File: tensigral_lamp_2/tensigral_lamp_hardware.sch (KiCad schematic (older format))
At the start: 95 parts, among them J1 USB_B_Micro, J2 JTAG, J3 DEVHDR, J4 WSOUT, J5 VPPS, J6 MICJ, J7 VDDS, J8 WS_SEL, P1 WSIN, P10 AUXTOUCH, P2 WSOUT, P3 VLED, P4 VLED, P5 GND, P6 GND, P9 TOPTOUCH, Q1 3404, Q2 3404, SW1 BOOT0, T1 TOUCH1, T2 TOUCH2, U1 STM32F042F4Px, U2 MT2492, U3 NUP4202, U4 XC6206P360MR, U5 LM321

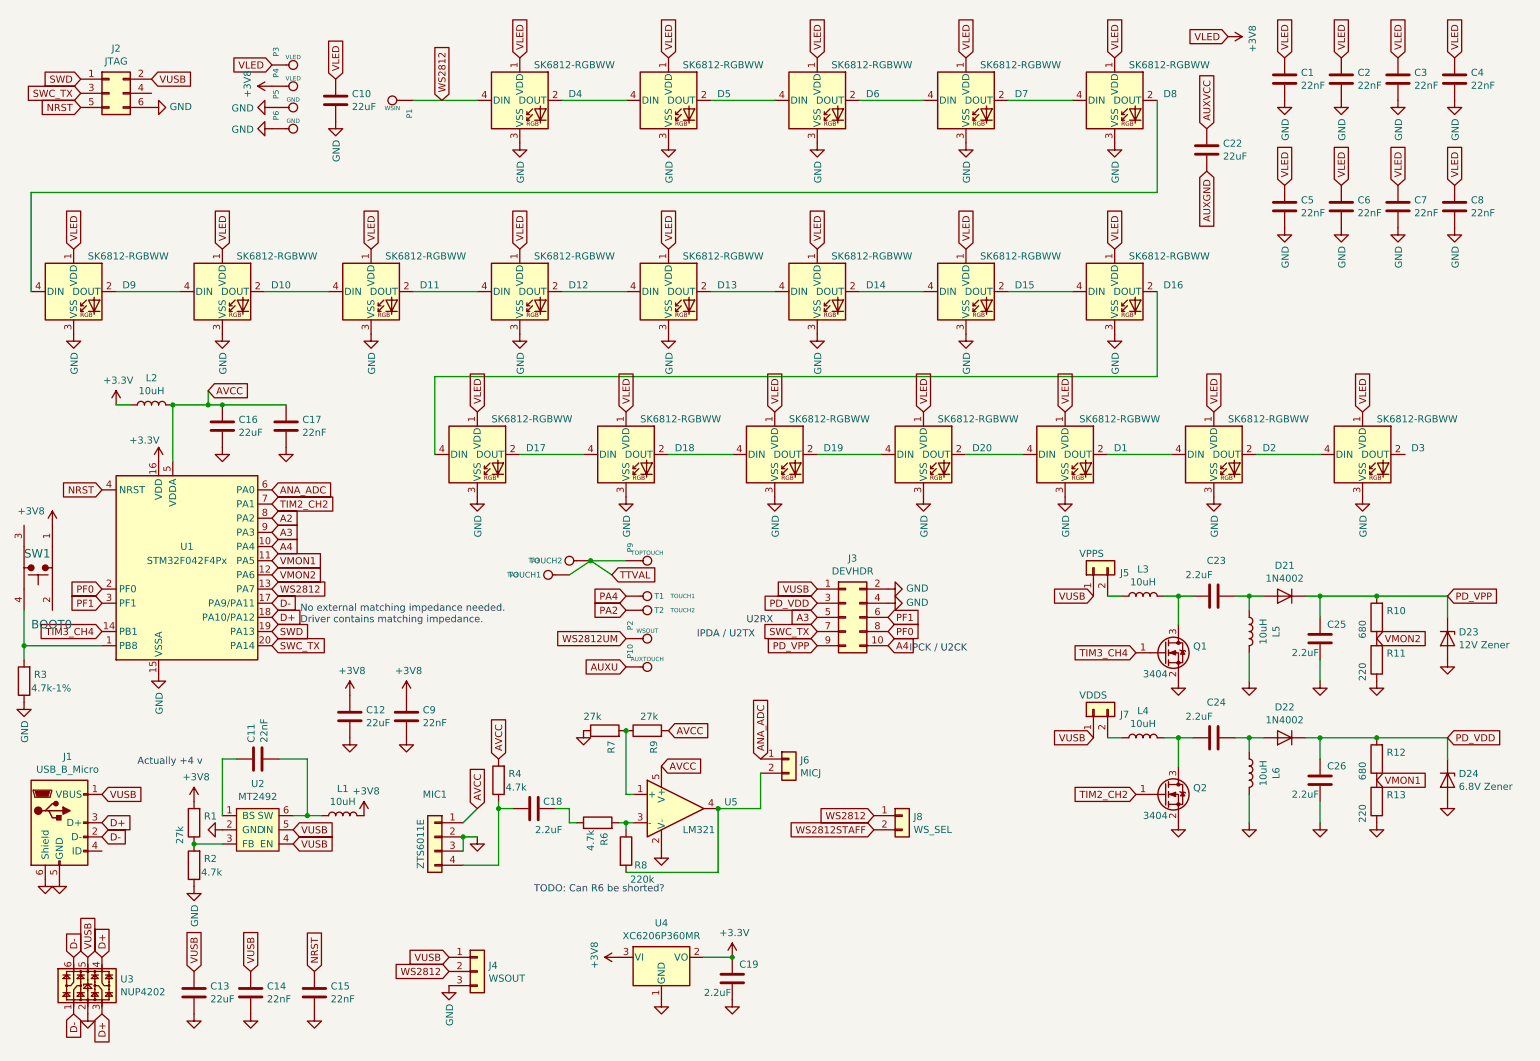
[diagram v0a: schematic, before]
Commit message: Bump
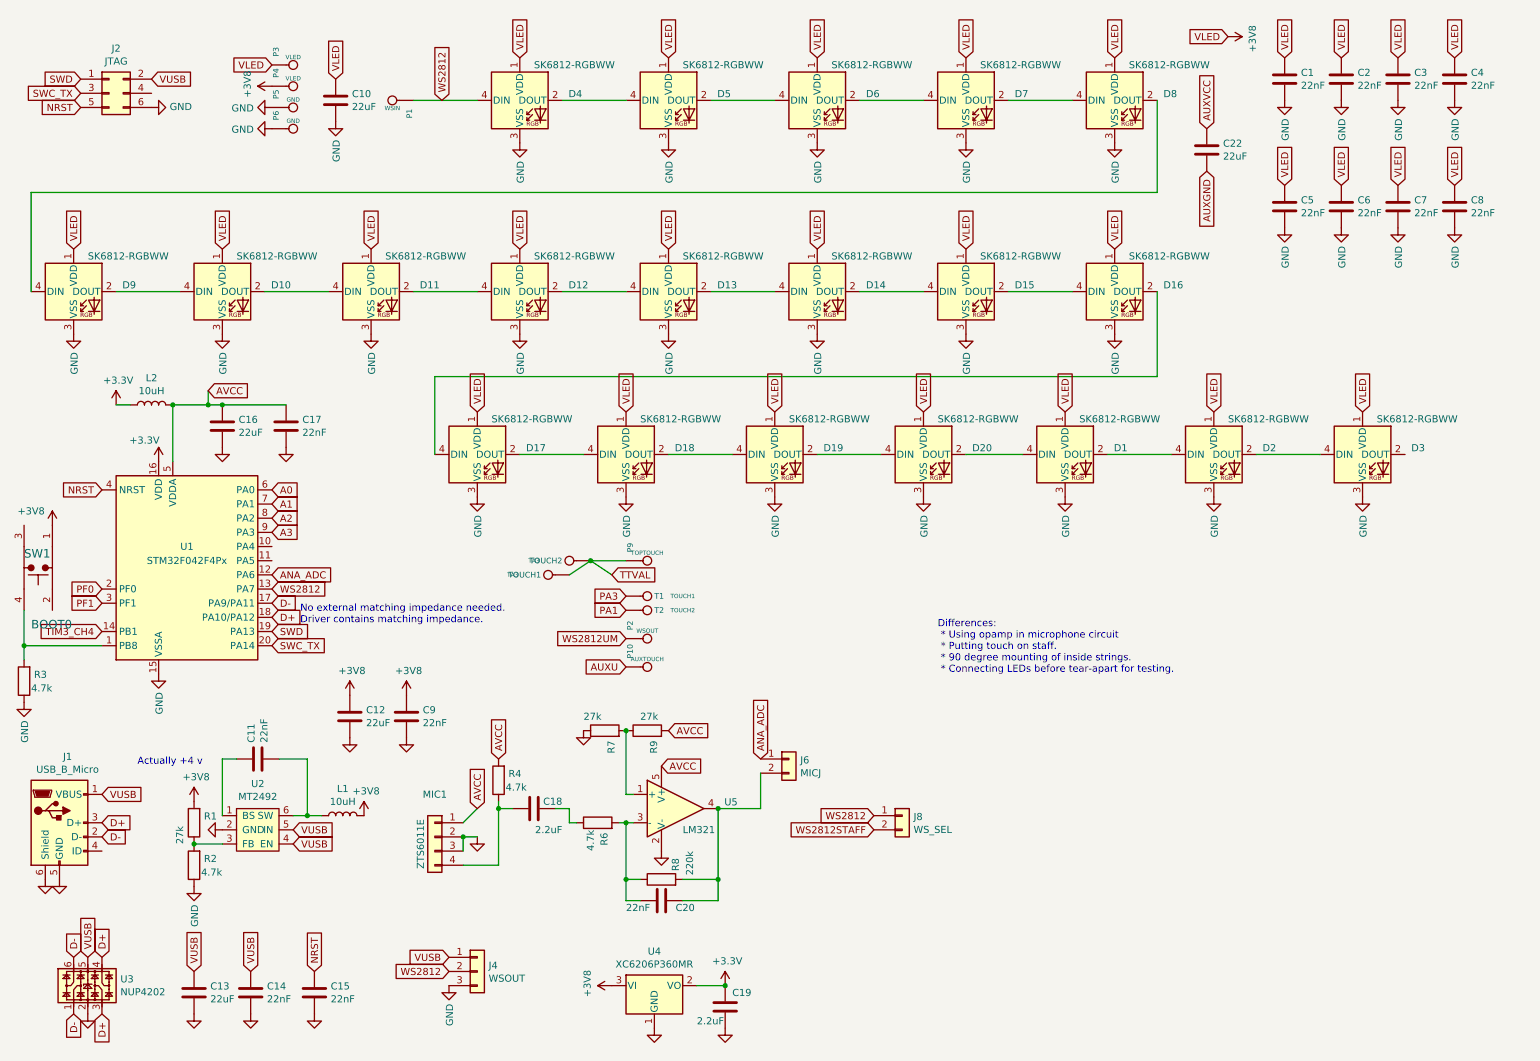
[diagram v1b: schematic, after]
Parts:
- removed C23, C24, C25, C26: 2.2uF, Capacitor_SMD:C_0805_2012Metric_Pad1.15x1.40mm_HandSolder, symbol tensigral_lamp_hardware-rescue:C-Device-tensigral_lamp_hardware-rescue
- removed D21, D22: 1N4002, Diode_SMD:D_SOD-123F, symbol Device:D
- removed D23: 12V Zener, Diode_SMD:D_SOD-123, symbol Device:D_Zener
- removed D24: 6.8V Zener, Diode_SMD:D_SOD-123, symbol Device:D_Zener
- removed J3: DEVHDR, Connector_PinSocket_2.54mm:PinSocket_2x05_P2.54mm_Vertical_SMD, symbol Connector_Generic:Conn_02x05_Odd_Even
- removed J5: VPPS, Jumper:SolderJumper-2_P1.3mm_Bridged_Pad1.0x1.5mm, symbol Connector_Generic:Conn_01x02
- removed J7: VDDS, Jumper:SolderJumper-2_P1.3mm_Bridged_Pad1.0x1.5mm, symbol Connector_Generic:Conn_01x02
- removed L3, L4, L5, L6: 10uH, Inductor_SMD:L_2816_7142Metric, symbol tensigral_lamp_hardware-rescue:L-Device-tensigral_lamp_hardware-rescue
- removed Q1, Q2: 3404, Package_TO_SOT_SMD:SOT-23, symbol Device:Q_NMOS_GSD
- removed R10, R12: 680, Resistor_SMD:R_0805_2012Metric_Pad1.15x1.40mm_HandSolder, symbol tensigral_lamp_hardware-rescue:R-Device-tensigral_lamp_hardware-rescue
- removed R11, R13: 220, Resistor_SMD:R_0805_2012Metric_Pad1.15x1.40mm_HandSolder, symbol tensigral_lamp_hardware-rescue:R-Device-tensigral_lamp_hardware-rescue
- added C20: 22nF, Capacitor_SMD:C_0805_2012Metric_Pad1.15x1.40mm_HandSolder, symbol tensigral_lamp_hardware-rescue:C-Device-tensigral_lamp_hardware-rescue
- R3: value 4.7k-1% -> 4.7k
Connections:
- net VMON2 is gone; now on net ANA_ADC: U1.12 (PA6)
- net ANA_ADC: no longer U1.6 (PA0)
- net at J6.2 (Pin_2), R8.2, U5.4: now also C20.1
- net at R6.2, R8.1, U5.3 (-): now also C20.2
- net A4: no longer names the net of U1.10 (PA4)
- net PA2 renamed PA1
- net PA4 renamed PA3
- net TIM2_CH2 renamed A1
- net VMON1: no longer names the net of U1.11 (PA5)
- new net A0: U1.6 (PA0)
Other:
- note added: "Differences:\n * Using opamp in microphone circuit\n * Putting touch on staff.\n * 90 degree mounting of inside strings.\n * Connecting LEDs before tear-apart for testing."
- note removed: "IPCK / U2CK\n"
- note removed: "IPDA / U2TX"
- note removed: "TODO: Can R6 be shorted?"
- note removed: "U2RX"
- moved on the sheet: C19, R8, U4
